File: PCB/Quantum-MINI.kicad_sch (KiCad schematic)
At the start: 85 parts, among them J2 Conn_01x06, J2 JTAG_TC2030, J3 USB_A, SW1 Boot, SW10 MX_SW_solder, SW11 MX_SW_HS, SW12 MX_SW_solder, SW13 MX_SW_HS, SW14 MX_SW_solder, SW15 MX_SW_HS, SW16 MX_SW_solder, SW17 MX_SW_HS, SW18 MX_SW_HS, SW19 MX_SW_solder, SW2 MX_SW_HS, SW20 MX_SW_solder, SW21 MX_SW_HS, SW22 MX_SW_HS, SW23 MX_SW_solder, SW24 MX_SW_HS, SW25 MX_SW_solder, SW26 MX_SW_solder, SW27 MX_SW_HS, SW28 MX_SW_HS, SW29 MX_SW_solder, SW3 MX_SW_solder, SW30 MX_SW_solder, SW31 MX_SW_HS, SW32 MX_SW_solder, SW33 MX_SW_HS, SW34 MX_SW_HS, SW35 MX_SW_solder, SW36 MX_SW_HS, SW37 MX_SW_solder, SW38 MX_SW_HS, SW39 MX_SW_solder, SW4 MX_SW_HS, SW40 MX_SW_HS, SW41 MX_SW_solder, SW42 SW_SPDT, SW5 MX_SW_solder, SW6 MX_SW_solder, SW7 MX_SW_HS, SW8 MX_SW_solder, SW9 MX_SW_HS, U1 XC6206, U2 USBLC6-2SC6, U3 RP2040, U4 W25Q128JVS, Y1 12MHz

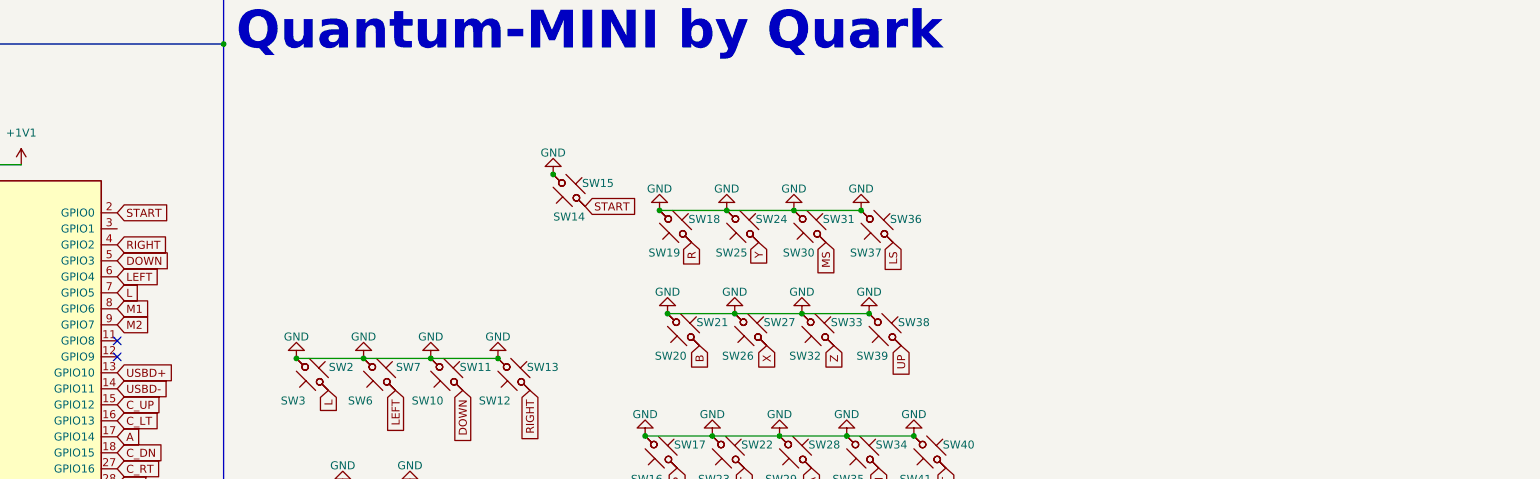
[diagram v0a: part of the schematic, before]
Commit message: Uploaded latest changes
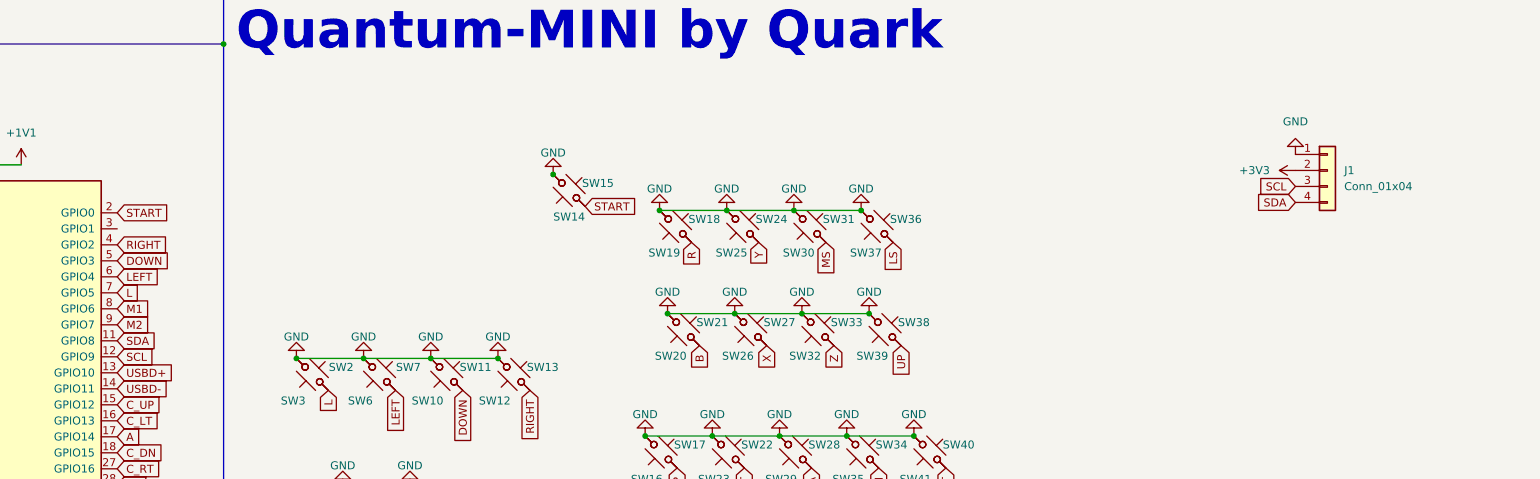
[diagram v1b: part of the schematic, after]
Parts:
- added J1: Conn_01x04, DevLibrary:SH1107, symbol Connector_Generic:Conn_01x04
- SW42: footprint Button_Switch_SMD:SW_SPDT_PCM12 -> Button_Switch_THT:SW_CuK_OS102011MA1QN1_SPDT_Angled
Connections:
- net +3V3: now also J1.2 (Pin_2)
- net GND: now also J1.1 (Pin_1)
- net SDA: now reaches U3.11 (GPIO8)
- net SDA: now also J1.4 (Pin_4)
- net SCL: now reaches U3.12 (GPIO9)
- net SCL: now also J1.3 (Pin_3)
- no-connect marks 4 -> 2
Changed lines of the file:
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@@
   )
   (no_connect (at 71.882 107.315))
-  (no_connect (at 71.882 71.755))
-  (no_connect (at 71.882 69.215))
   (no_connect (at 71.882 126.365))
   (wire (pts (xy 327.787 162.179) (xy 334.391 162.179))
@@
     )
   )
+  (global_label "SDA" (shape input) (at 71.882 69.215 0) (fields_autoplaced)
+    (effects (font (size 1.27 1.27)) (justify left))
+    (property "Intersheetrefs" "${INTERSHEET_REFS}" (at 78.3559 69.215 0)
+      (effects (font (size 1.27 1.27)) (justify left) hide)
+    )
+  )
   (global_label "LS" (shape input) (at 195.072 53.594 270) (fields_autoplaced)
     (effects (font (size 1.27 1.27)) (justify right))
@@
     )
   )
+  (global_label "SCL" (shape input) (at 258.953 44.704 180) (fields_autoplaced)
+    (effects (font (size 1.27 1.27)) (justify right))
+    (property "Intersheetrefs" "${INTERSHEET_REFS}" (at 252.5396 44.704 0)
+      (effects (font (size 1.27 1.27)) (justify right) hide)
+    )
+  )
   (global_label "SD1" (shape input) (at 31.242 118.745 180) (fields_autoplaced)
     (effects (font (size 1.27 1.27)) (justify right))
@@
     )
   )
+  (global_label "SCL" (shape input) (at 71.882 71.755 0) (fields_autoplaced)
+    (effects (font (size 1.27 1.27)) (justify left))
+    (property "Intersheetrefs" "${INTERSHEET_REFS}" (at 78.2954 71.755 0)
+      (effects (font (size 1.27 1.27)) (justify left) hide)
+    )
+  )
   (global_label "SD1" (shape input) (at 359.791 162.179 0) (fields_autoplaced)
     (effects (font (size 1.27 1.27)) (justify left))
@@
     )
   )
+  (global_label "SDA" (shape input) (at 258.953 47.244 180) (fields_autoplaced)
+    (effects (font (size 1.27 1.27)) (justify right))
+    (property "Intersheetrefs" "${INTERSHEET_REFS}" (at 252.4791 47.244 0)
+      (effects (font (size 1.27 1.27)) (justify right) hide)
+    )
+  )
   (global_label "START" (shape input) (at 71.882 48.895 0) (fields_autoplaced)
     (effects (font (size 1.27 1.27)) (justify left))
@@
     )
   )
+  (symbol (lib_name "+3V3_1") (lib_id "power:+3V3") (at 258.953 42.164 90) (unit 1)
+    (in_bom yes) (on_board yes) (dnp no) (fields_autoplaced)
+    (property "Reference" "#PWR015" (at 262.763 42.164 0)
+      (effects (font (size 1.27 1.27)) hide)
+    )
+    (property "Value" "+3V3" (at 254.889 42.164 90)
+      (effects (font (size 1.27 1.27)) (justify left))
+    )
+    (property "Footprint" "" (at 258.953 42.164 0)
+      (effects (font (size 1.27 1.27)) hide)
+    )
+    (property "Datasheet" "" (at 258.953 42.164 0)
+      (effects (font (size 1.27 1.27)) hide)
+    )
+    (pin "1")
+    (instances
+      (project "Quantum-MINI"
+        (path "/9aaaec2c-dd67-47a8-8e5a-58d136f523d5"
+          (reference "#PWR015") (unit 1)
+        )
+      )
+    )
+  )
   (symbol (lib_id "Device:C_Small") (at 39.497 184.15 0) (unit 1)
     (in_bom yes) (on_board yes) (dnp no)
@@
     )
   )
+  (symbol (lib_id "Connector_Generic:Conn_01x04") (at 264.033 42.164 0) (unit 1)
+    (in_bom yes) (on_board yes) (dnp no) (fields_autoplaced)
+    (property "Reference" "J1" (at 266.7 42.164 0)
+      (effects (font (size 1.27 1.27)) (justify left))
+    )
+    (property "Value" "Conn_01x04" (at 266.7 44.704 0)
+      (effects (font (size 1.27 1.27)) (justify left))
+    )
+    (property "Footprint" "DevLibrary:SH1107" (at 264.033 42.164 0)
+      (effects (font (size 1.27 1.27)) hide)
+    )
+    (property "Datasheet" "~" (at 264.033 42.164 0)
+      (effects (font (size 1.27 1.27)) hide)
+    )
+    (pin "1")
+    (pin "2")
+    (pin "3")
+    (pin "4")
+    (instances
+      (project "Quantum-MINI"
+        (path "/9aaaec2c-dd67-47a8-8e5a-58d136f523d5"
+          (reference "J1") (unit 1)
+        )
+      )
+    )
+  )
   (symbol (lib_id "marbastlib-mx:MX_SW_HS") (at 168.91 86.868 0) (unit 1)
     (in_bom yes) (on_board yes) (dnp no)
@@
     )
   )
+  (symbol (lib_name "GND_2") (lib_id "power:GND") (at 258.953 39.624 180) (unit 1)
+    (in_bom yes) (on_board yes) (dnp no) (fields_autoplaced)
+    (property "Reference" "#PWR014" (at 258.953 33.274 0)
+      (effects (font (size 1.27 1.27)) hide)
+    )
+    (property "Value" "GND" (at 258.953 34.417 0)
+      (effects (font (size 1.27 1.27)))
+    )
+    (property "Footprint" "" (at 258.953 39.624 0)
+      (effects (font (size 1.27 1.27)) hide)
+    )
+    (property "Datasheet" "" (at 258.953 39.624 0)
+      (effects (font (size 1.27 1.27)) hide)
+    )
+    (pin "1")
+    (instances
+      (project "Quantum-MINI"
+        (path "/9aaaec2c-dd67-47a8-8e5a-58d136f523d5"
+          (reference "#PWR014") (unit 1)
+        )
+      )
+    )
+  )
   (symbol (lib_id "power:+3V3") (at 27.3492 42.545 0) (unit 1)
     (in_bom yes) (on_board yes) (dnp no)
@@
       (effects (font (size 1.27 1.27)))
     )
-    (property "Footprint" "Button_Switch_SMD:SW_SPDT_PCM12" (at 326.898 205.359 0)
+    (property "Footprint" "Button_Switch_THT:SW_CuK_OS102011MA1QN1_SPDT_Angled" (at 326.898 205.359 0)
       (effects (font (size 1.27 1.27)) hide)
     )
